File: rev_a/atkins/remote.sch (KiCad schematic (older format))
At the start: 19 parts, among them J1 UARTSCREW, J10 Conn_01x04_Female, J11 BME390, J12 UARTPINS, J13 Conn_01x04_Female, J2 UARTPINS, J3 UARTSCREW, J4 Screw_Terminal_01x04, J5 Conn_01x02_Female, J6 Conn_01x12_Male, J7 Conn_01x16_Female, J8 Screw_Terminal_01x02, J9 SCD30

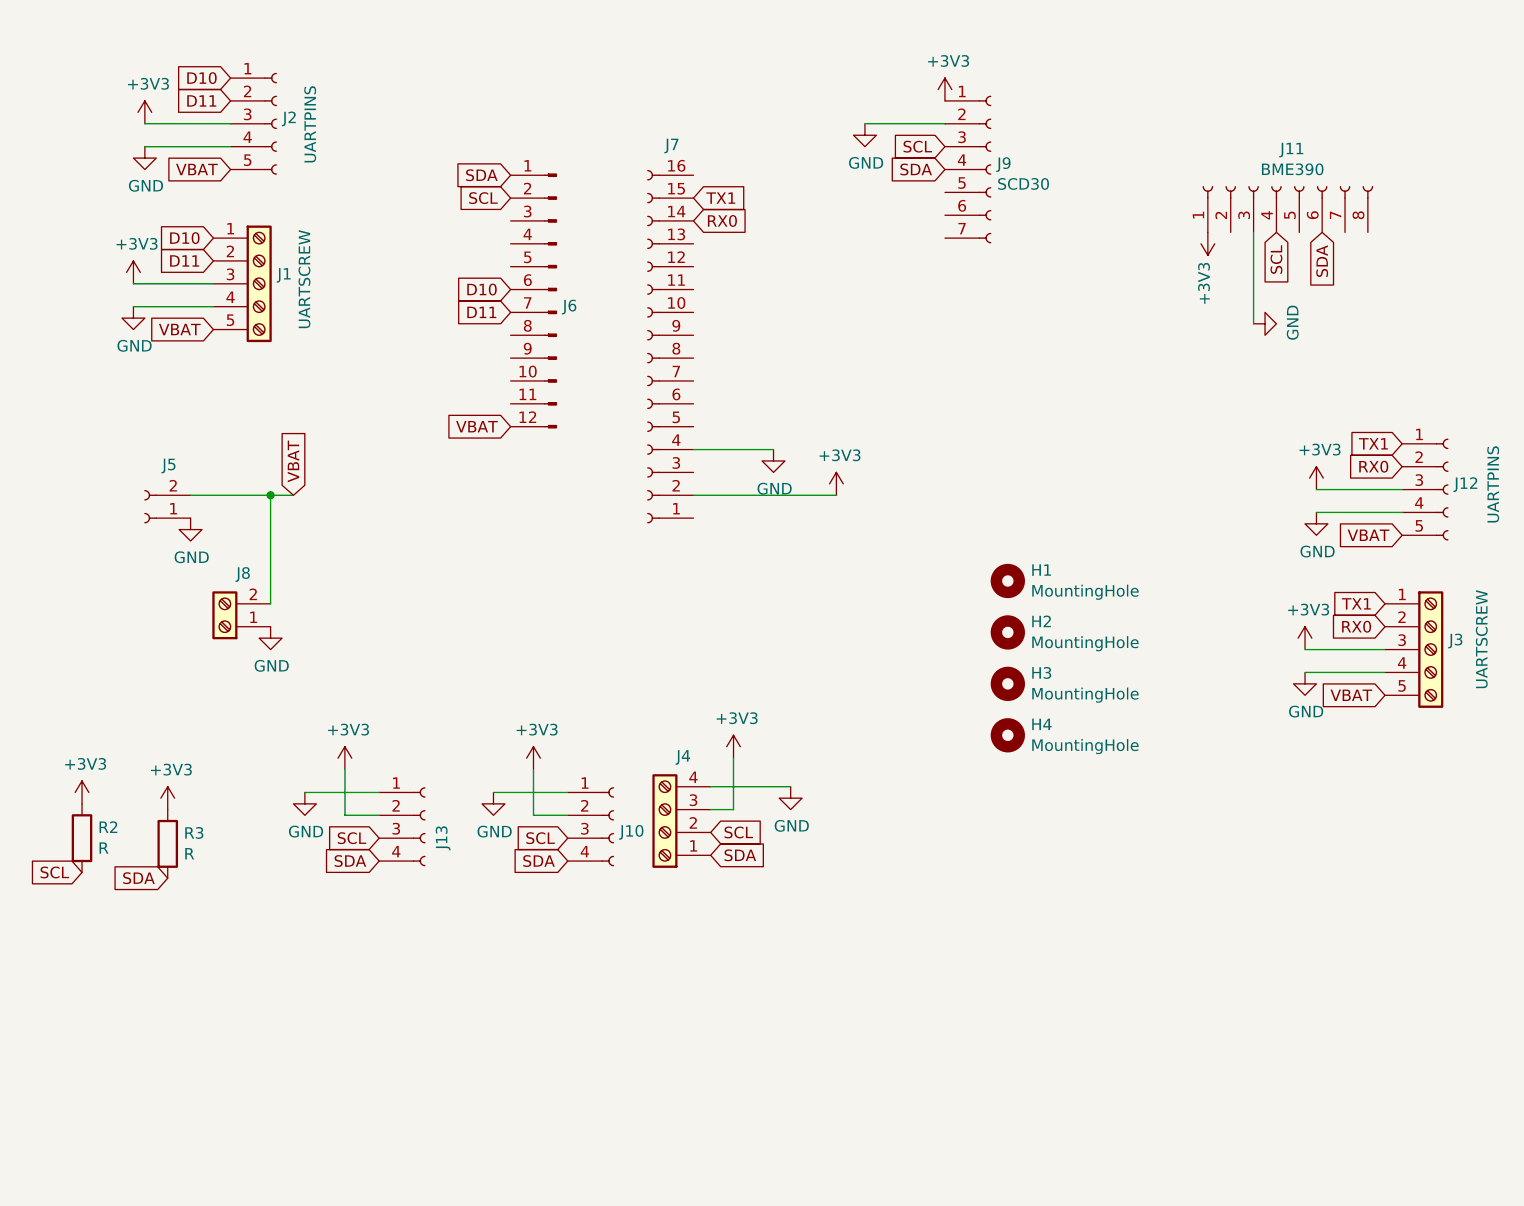
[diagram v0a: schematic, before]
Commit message: update
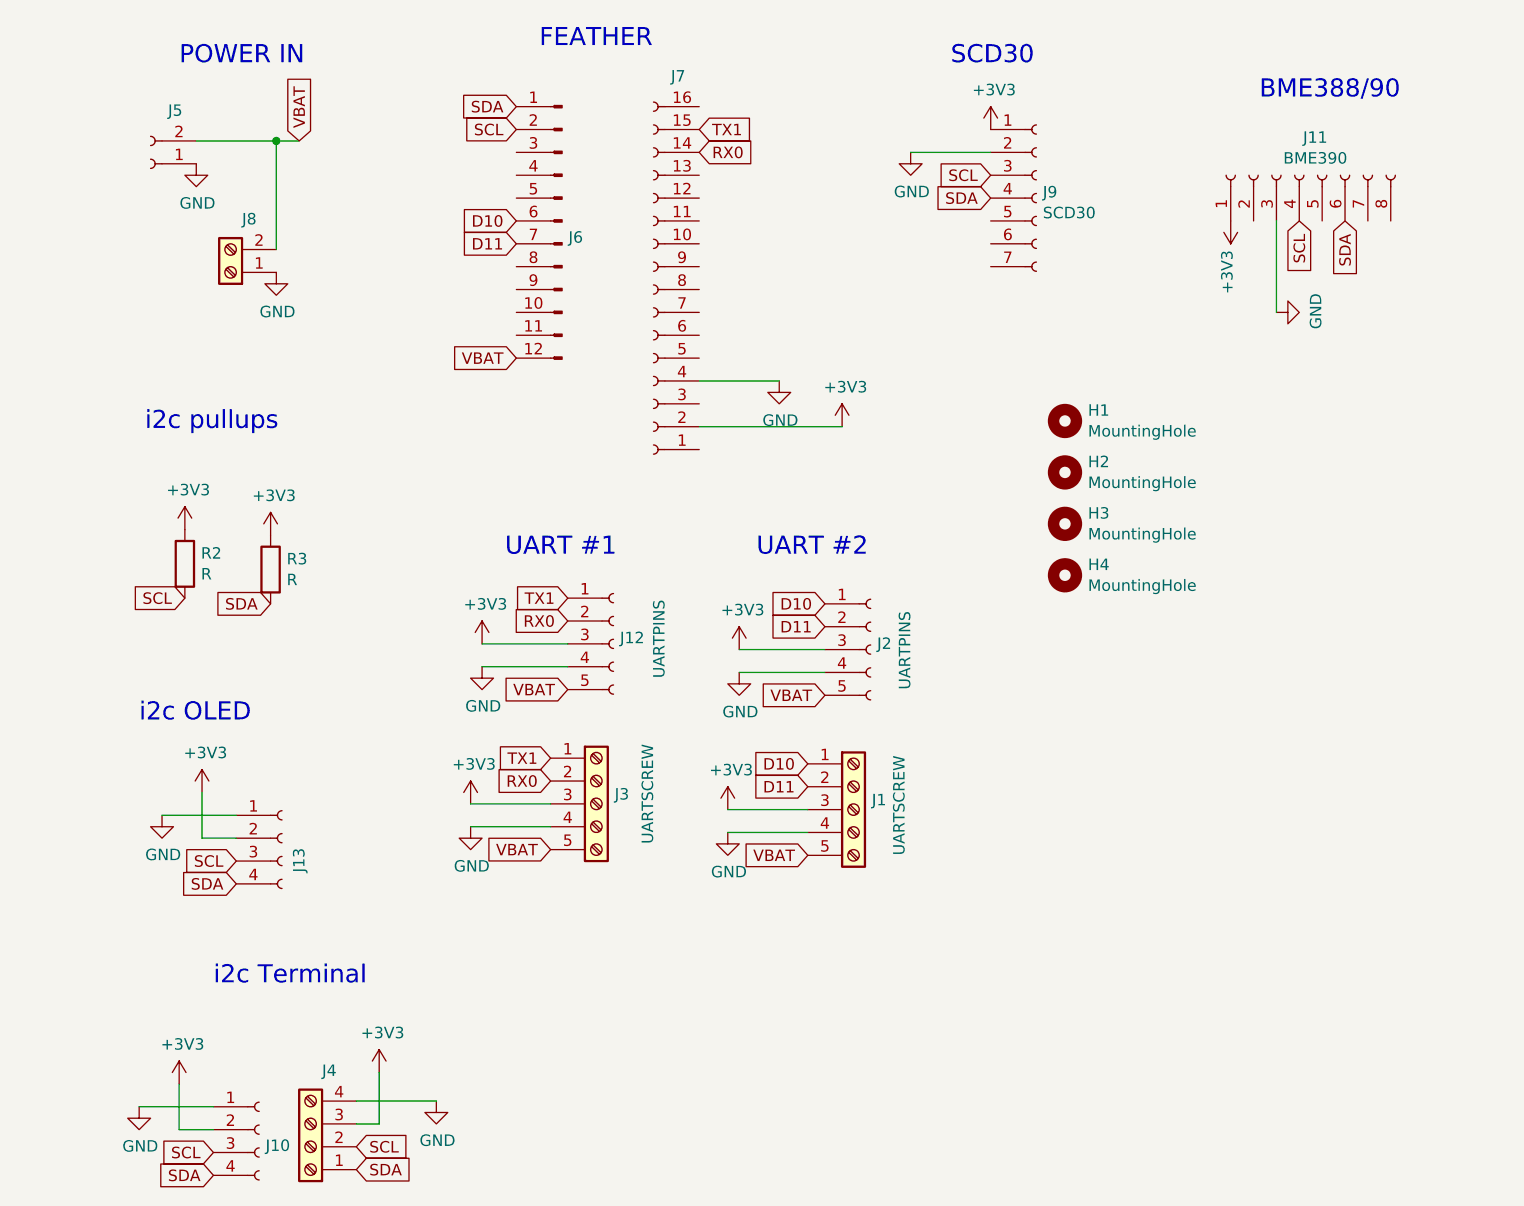
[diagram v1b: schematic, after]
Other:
- note added: "BME388/90"
- note added: "FEATHER"
- note added: "POWER IN"
- note added: "SCD30"
- note added: "UART #1"
- note added: "UART #2"
- note added: "i2c OLED"
- note added: "i2c Terminal"
- note added: "i2c pullups"
- moved on the sheet: H1, H2, H3, H4, J1, J10, J11, J12, J13, J2, J3, J4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
